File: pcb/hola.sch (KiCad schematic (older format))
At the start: 35 parts, among them J1 USB_B, J2 USB_B_Micro, J3 Conn_01x08, J4 Conn_01x02, Q1 DTB123T, U1 TPS61090, U2 MCP73871

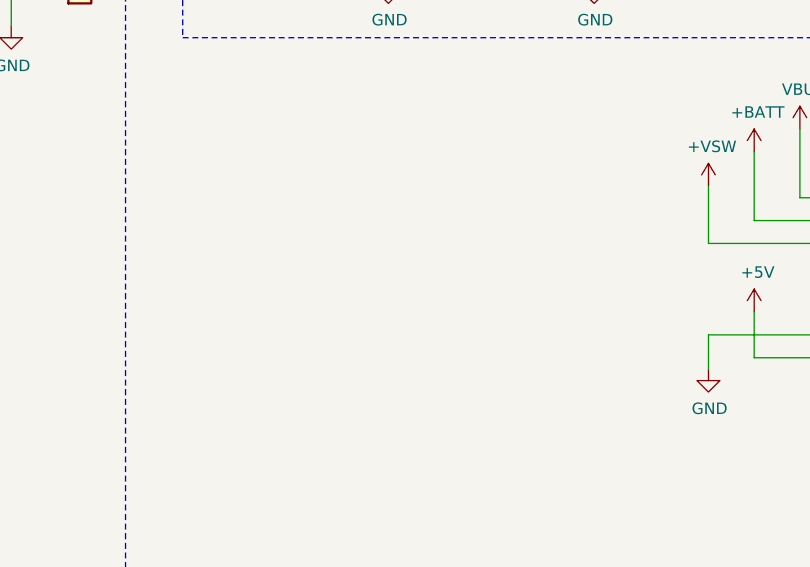
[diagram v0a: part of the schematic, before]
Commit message: actualizacion
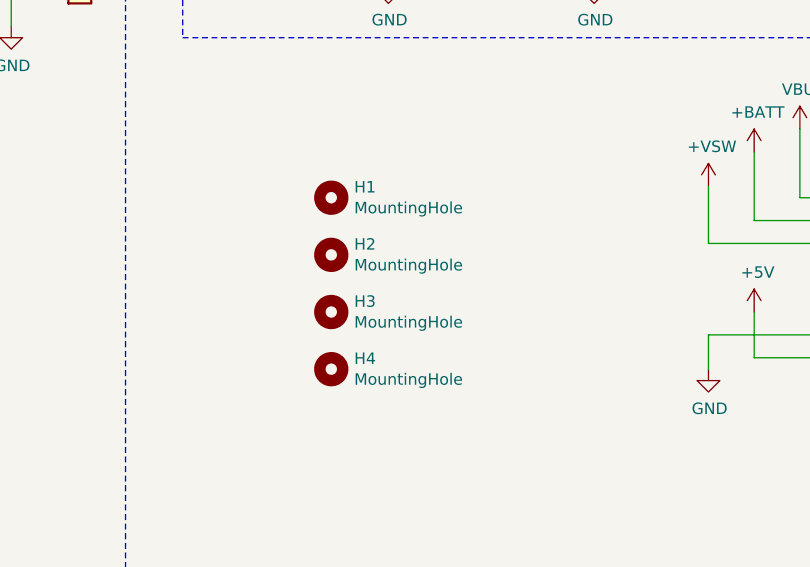
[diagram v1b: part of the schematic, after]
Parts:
- added H1, H2, H3, H4: MountingHole, MountingHole:MountingHole_2.1mm, symbol Mechanical:MountingHole
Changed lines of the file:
@@
 Wire Wire Line
 	8100 3900 8100 4300
+$Comp
+L Mechanical:MountingHole H1
+U 1 1 61700954
+P 6950 5250
+F 0 "H1" H 7050 5296 50  0000 L CNN
+F 1 "MountingHole" H 7050 5205 50  0000 L CNN
+F 2 "MountingHole:MountingHole_2.1mm" H 6950 5250 50  0001 C CNN
+F 3 "~" H 6950 5250 50  0001 C CNN
+	1    6950 5250
+	1    0    0    -1
+$EndComp
+$Comp
+L Mechanical:MountingHole H2
+U 1 1 617012D8
+P 6950 5500
+F 0 "H2" H 7050 5546 50  0000 L CNN
+F 1 "MountingHole" H 7050 5455 50  0000 L CNN
+F 2 "MountingHole:MountingHole_2.1mm" H 6950 5500 50  0001 C CNN
+F 3 "~" H 6950 5500 50  0001 C CNN
+	1    6950 5500
+	1    0    0    -1
+$EndComp
+$Comp
+L Mechanical:MountingHole H3
+U 1 1 61701D3B
+P 6950 5750
+F 0 "H3" H 7050 5796 50  0000 L CNN
+F 1 "MountingHole" H 7050 5705 50  0000 L CNN
+F 2 "MountingHole:MountingHole_2.1mm" H 6950 5750 50  0001 C CNN
+F 3 "~" H 6950 5750 50  0001 C CNN
+	1    6950 5750
+	1    0    0    -1
+$EndComp
+$Comp
+L Mechanical:MountingHole H4
+U 1 1 61702385
+P 6950 6000
+F 0 "H4" H 7050 6046 50  0000 L CNN
+F 1 "MountingHole" H 7050 5955 50  0000 L CNN
+F 2 "MountingHole:MountingHole_2.1mm" H 6950 6000 50  0001 C CNN
+F 3 "~" H 6950 6000 50  0001 C CNN
+	1    6950 6000
+	1    0    0    -1
+$EndComp
 $EndSCHEMATC

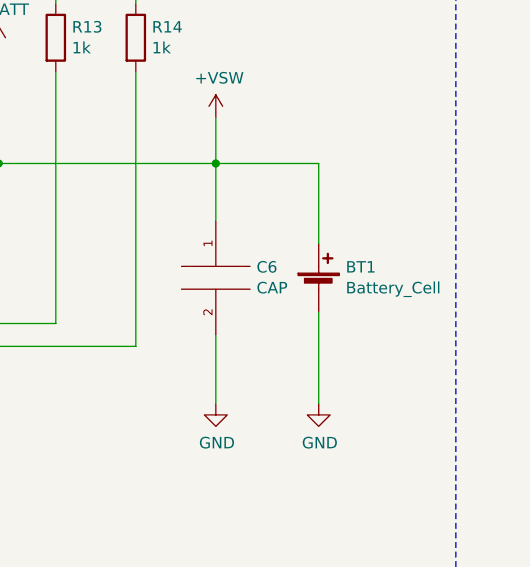
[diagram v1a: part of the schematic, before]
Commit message: actualizacion
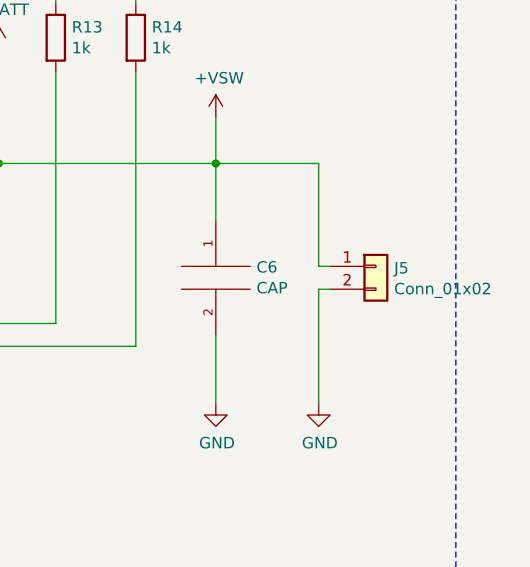
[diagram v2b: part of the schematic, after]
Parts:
- removed BT1: Battery_Cell, Battery:BatteryHolder_Keystone_3000_1x12mm, symbol Device:Battery_Cell
- added J5: Conn_01x02, Connector_JST:JST_PH_S2B-PH-K_1x02_P2.00mm_Horizontal, symbol Connector_Generic:Conn_01x02
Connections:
- net +VSW: now also J5.1 (Pin_1)
- net GND: now also J5.2 (Pin_2)
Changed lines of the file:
@@
-$EndComp
-$Comp
-L Device:Battery_Cell BT1
-U 1 1 6146719E
-P 10300 3250
-F 0 "BT1" H 10418 3346 50  0000 L CNN
-F 1 "Battery_Cell" H 10418 3255 50  0000 L CNN
-F 2 "Battery:BatteryHolder_Keystone_3000_1x12mm" V 10300 3310 50  0001 C CNN
-F 3 "https://www.mouser.com/Power/Battery-Holders-Clips-Contacts/Datasheets/_/N-cicxg?keyword=534-104" V 10300 3310 50  0001 C CNN
-	1    10300 3250
-	1    0    0    -1
 $EndComp
 $Comp
@@
 $EndComp
 Wire Wire Line
-	10300 3350 10300 3750
-Wire Wire Line
 	9850 3450 9850 3750
-Wire Wire Line
-	10300 3050 10300 2700
-Wire Wire Line
-	10300 2700 9850 2700
 Wire Wire Line
 	9850 2700 9850 2950
@@
 	1    0    0    -1
 $EndComp
+$Comp
+L Connector_Generic:Conn_01x02 J5
+U 1 1 6172C34A
+P 10550 3150
+F 0 "J5" H 10630 3142 50  0000 L CNN
+F 1 "Conn_01x02" H 10630 3051 50  0000 L CNN
+F 2 "Connector_JST:JST_PH_S2B-PH-K_1x02_P2.00mm_Horizontal" H 10550 3150 50  0001 C CNN
+F 3 "~" H 10550 3150 50  0001 C CNN
+	1    10550 3150
+	1    0    0    -1
+$EndComp
+Wire Wire Line
+	10300 3750 10300 3250
+Wire Wire Line
+	10300 3250 10350 3250
+Wire Wire Line
+	10350 3150 10300 3150
+Wire Wire Line
+	10300 3150 10300 2700
+Wire Wire Line
+	10300 2700 9850 2700
 $EndSCHEMATC
